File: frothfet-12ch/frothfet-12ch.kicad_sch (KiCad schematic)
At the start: 8 parts

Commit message: more pre-production tweaks
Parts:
- U1: footprint (none) -> yarrboard:Waveshare-ESP32-S3-dev-kit
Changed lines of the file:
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@@
 			)
 		)
-		(property "Footprint" ""
+		(property "Footprint" "yarrboard:Waveshare-ESP32-S3-dev-kit"
 			(at 139.7 54.61 0)
 			(effects

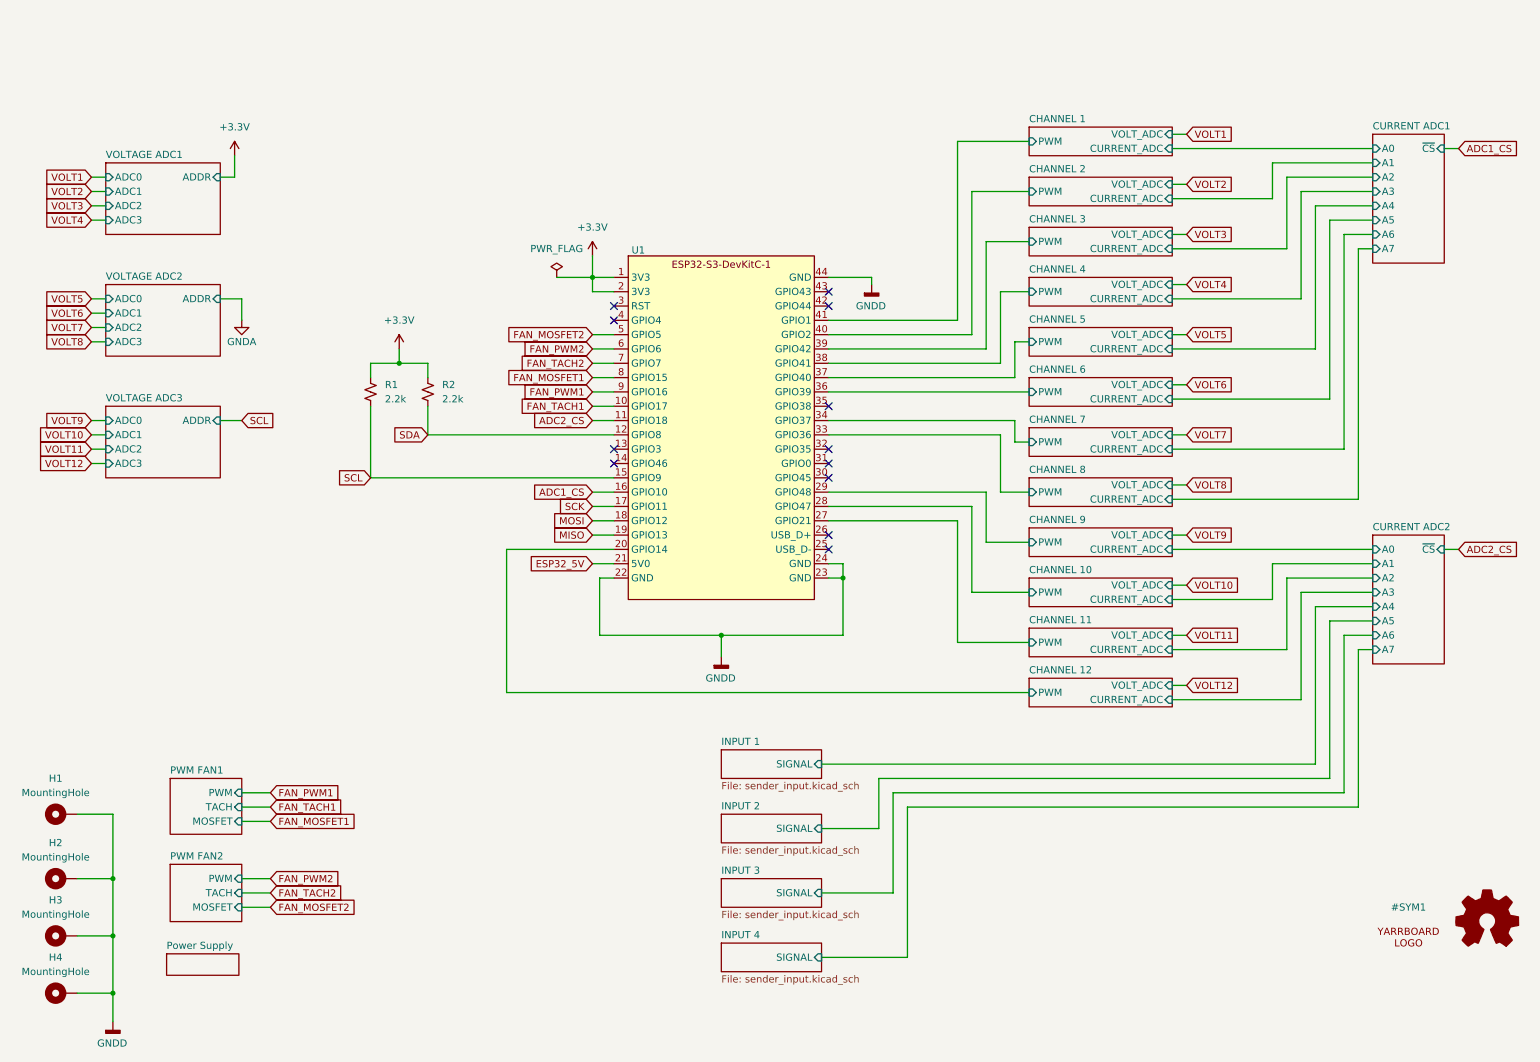
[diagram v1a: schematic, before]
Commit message: lots of big updates
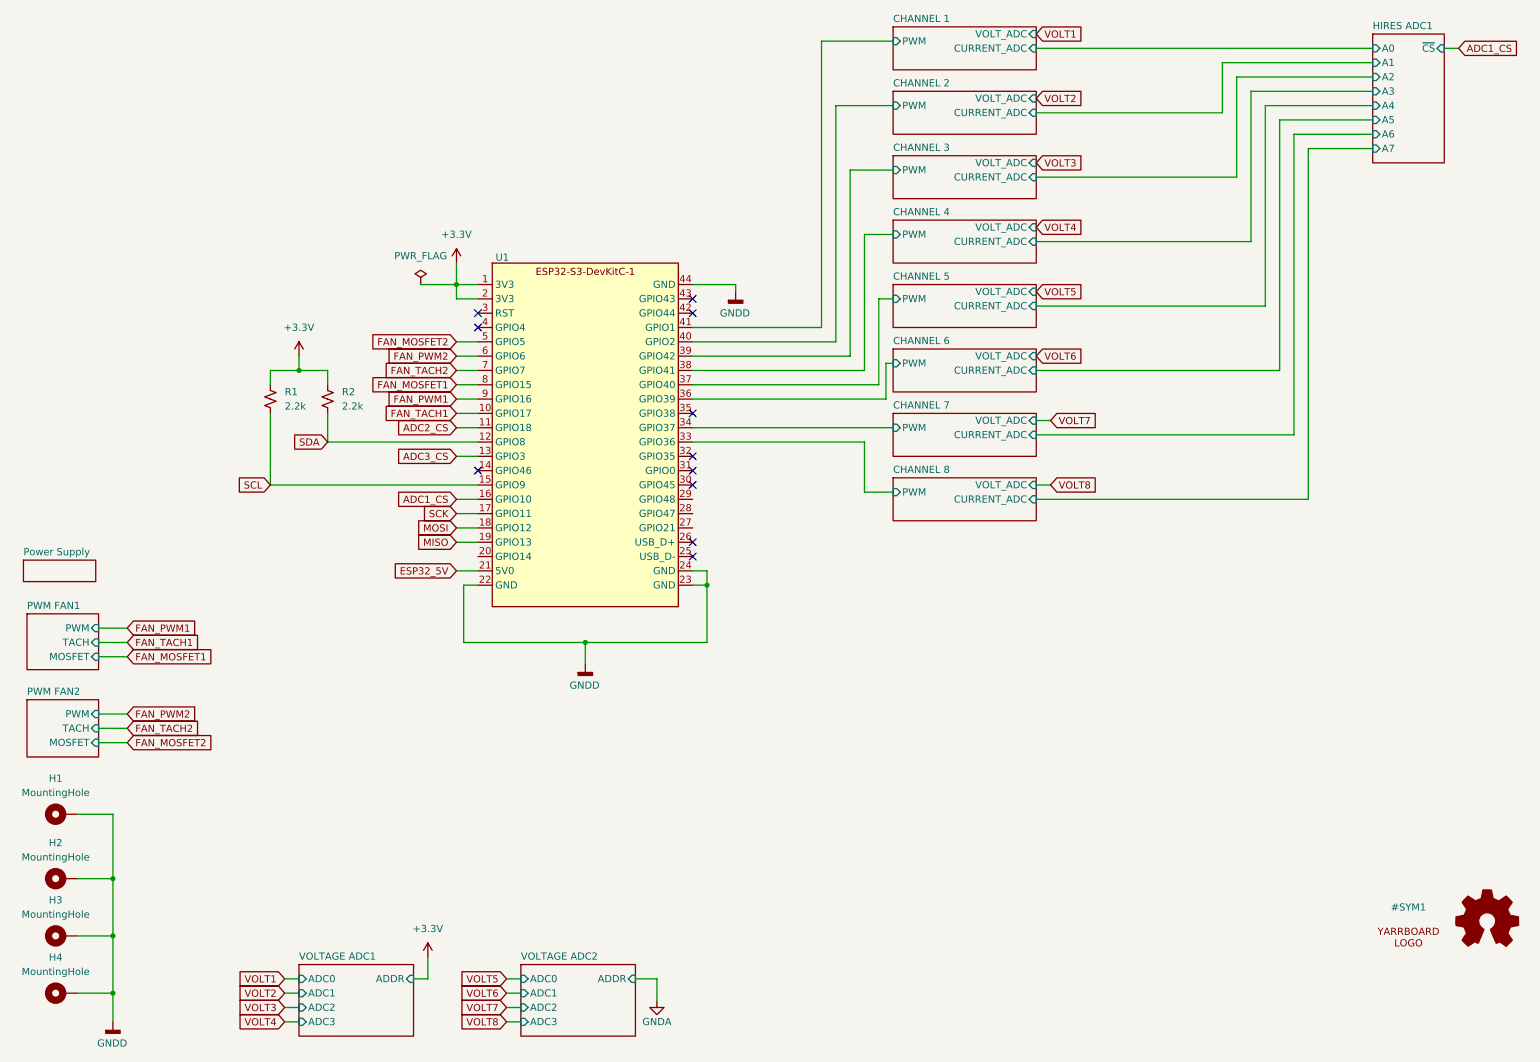
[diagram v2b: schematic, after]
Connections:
- net ADC3_CS: now reaches U1.13 (GPIO3)
- net CHANNEL 10/PWM: no longer names the net of U1.28 (GPIO47)
- net CHANNEL 11/PWM: no longer names the net of U1.27 (GPIO21)
- net CHANNEL 12/PWM: no longer names the net of U1.20 (GPIO14)
- net CHANNEL 9/PWM: no longer names the net of U1.29 (GPIO48)
- no-connect marks 12 -> 11
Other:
- sheet CURRENT ADC1 renamed HIRES ADC1
- removed sheet CHANNEL 10
- removed sheet CHANNEL 11
- removed sheet CHANNEL 12
- removed sheet CHANNEL 9
- removed sheet CURRENT ADC2
- removed sheet INPUT 1
- removed sheet INPUT 2
- removed sheet INPUT 3
- removed sheet INPUT 4
- removed sheet VOLTAGE ADC3
- moved on the sheet: R1, R2, U1
